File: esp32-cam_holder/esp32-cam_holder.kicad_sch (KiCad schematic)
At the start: 5 parts, among them J1 RJ45_Shielded, J2 Conn_01x03_Pin, U1 ESP32-CAM

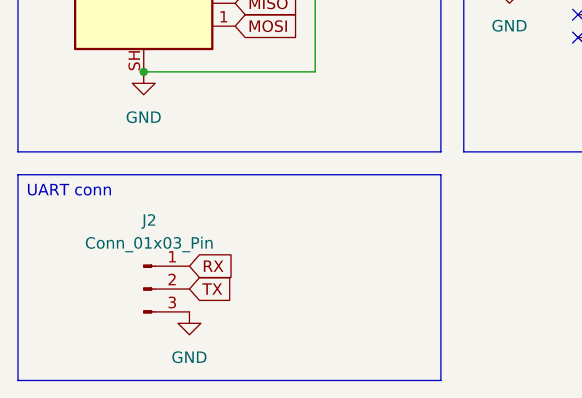
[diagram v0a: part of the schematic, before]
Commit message: update
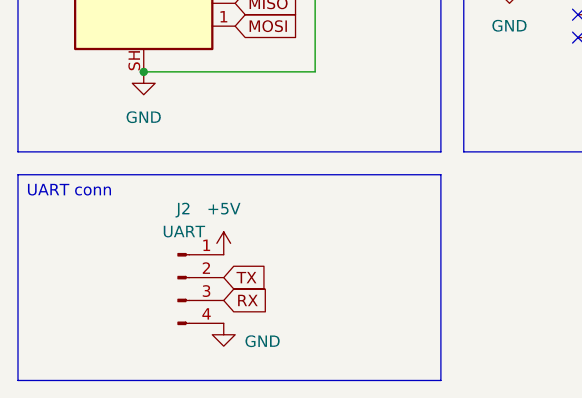
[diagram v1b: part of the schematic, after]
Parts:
- removed J2: Conn_01x03_Pin, Connector_PinHeader_2.54mm:PinHeader_1x03_P2.54mm_Horizontal, symbol Connector:Conn_01x03_Pin
- added J2: UART, Connector_PinHeader_2.54mm:PinHeader_1x04_P2.54mm_Horizontal, symbol Connector:Conn_01x04_Pin
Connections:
- net +5V: now also J2.1 (Pin_1)
- net GND: now also J2.4 (Pin_4)
- net RX: now also J2.3 (Pin_3)
- net TX: now also J2.2 (Pin_2)
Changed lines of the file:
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@@
+		)
+	)
+	(global_label "TX"
+		(shape input)
+		(at 36.83 71.12 0)
+		(fields_autoplaced yes)
+		(effects
+			(font
+				(size 1.27 1.27)
+			)
+			(justify left)
+		)
+		(property "Intersheetrefs" "${INTERSHEET_REFS}"
+			(at 41.9923 71.12 0)
+			(hide yes)
+			(show_name no)
+			(do_not_autoplace no)
+			(effects
+				(font
+					(size 1.27 1.27)
+				)
+				(justify left)
+			)
 		)
 	)
@@
 		)
 	)
-	(global_label "RX"
+	(global_label "MISO"
 		(shape input)
-		(at 33.02 69.85 0)
+		(at 38.1 40.64 0)
 		(fields_autoplaced yes)
 		(effects
@@
 		)
 		(property "Intersheetrefs" "${INTERSHEET_REFS}"
-			(at 38.4847 69.85 0)
+			(at 45.6814 40.64 0)
 			(hide yes)
 			(show_name no)
@@
 	(global_label "MISO"
 		(shape input)
-		(at 38.1 40.64 0)
+		(at 111.76 39.37 0)
 		(fields_autoplaced yes)
 		(effects
@@
 		)
 		(property "Intersheetrefs" "${INTERSHEET_REFS}"
-			(at 45.6814 40.64 0)
+			(at 119.3414 39.37 0)
 			(hide yes)
 			(show_name no)
@@
 		)
 	)
-	(global_label "MISO"
+	(global_label "TX"
 		(shape input)
-		(at 111.76 39.37 0)
+		(at 76.2 29.21 180)
 		(fields_autoplaced yes)
 		(effects
@@
 				(size 1.27 1.27)
 			)
-			(justify left)
+			(justify right)
 		)
 		(property "Intersheetrefs" "${INTERSHEET_REFS}"
-			(at 119.3414 39.37 0)
-			(hide yes)
-			(show_name no)
-			(do_not_autoplace no)
-			(effects
-				(font
-					(size 1.27 1.27)
-				)
-				(justify left)
-			)
-		)
-	)
-	(global_label "TX"
+			(at 71.0377 29.21 0)
+			(hide yes)
+			(show_name no)
+			(do_not_autoplace no)
+			(effects
+				(font
+					(size 1.27 1.27)
+				)
+				(justify right)
+			)
+		)
+	)
+	(global_label "RX"
 		(shape input)
-		(at 76.2 29.21 180)
+		(at 36.83 73.66 0)
 		(fields_autoplaced yes)
 		(effects
@@
 				(size 1.27 1.27)
 			)
-			(justify right)
+			(justify left)
 		)
 		(property "Intersheetrefs" "${INTERSHEET_REFS}"
-			(at 71.0377 29.21 0)
-			(hide yes)
-			(show_name no)
-			(do_not_autoplace no)
-			(effects
-				(font
-					(size 1.27 1.27)
-				)
-				(justify right)
+			(at 42.2947 73.66 0)
+			(hide yes)
+			(show_name no)
+			(do_not_autoplace no)
+			(effects
+				(font
+					(size 1.27 1.27)
+				)
+				(justify left)
 			)
 		)
@@
 		(property "Intersheetrefs" "${INTERSHEET_REFS}"
 			(at 126.0542 34.29 0)
-			(hide yes)
-			(show_name no)
-			(do_not_autoplace no)
-			(effects
-				(font
-					(size 1.27 1.27)
-				)
-				(justify left)
-			)
-		)
-	)
-	(global_label "TX"
-		(shape input)
-		(at 33.02 72.39 0)
-		(fields_autoplaced yes)
-		(effects
-			(font
-				(size 1.27 1.27)
-			)
-			(justify left)
-		)
-		(property "Intersheetrefs" "${INTERSHEET_REFS}"
-			(at 38.1823 72.39 0)
 			(hide yes)
 			(show_name no)
@@
 	)
 	(symbol
-		(lib_id "Connector:Conn_01x03_Pin")
-		(at 27.94 72.39 0)
+		(lib_id "Connector:Conn_01x04_Pin")
+		(at 31.75 71.12 0)
 		(unit 1)
 		(body_style 1)
@@
 		(fields_autoplaced yes)
 		(property "Reference" "J2"
-			(at 28.575 64.77 0)
-			(show_name no)
-			(do_not_autoplace no)
-			(effects
-				(font
-					(size 1.27 1.27)
-				)
-			)
-		)
-		(property "Value" "Conn_01x03_Pin"
-			(at 28.575 67.31 0)
-			(show_name no)
-			(do_not_autoplace no)
-			(effects
-				(font
-					(size 1.27 1.27)
-				)
-			)
-		)
-		(property "Footprint" "Connector_PinHeader_2.54mm:PinHeader_1x03_P2.54mm_Horizontal"
-			(at 27.94 72.39 0)
+			(at 32.385 63.5 0)
+			(show_name no)
+			(do_not_autoplace no)
+			(effects
+				(font
+					(size 1.27 1.27)
+				)
+			)
+		)
+		(property "Value" "UART"
+			(at 32.385 66.04 0)
+			(show_name no)
+			(do_not_autoplace no)
+			(effects
+				(font
+					(size 1.27 1.27)
+				)
+			)
+		)
+		(property "Footprint" "Connector_PinHeader_2.54mm:PinHeader_1x04_P2.54mm_Horizontal"
+			(at 31.75 71.12 0)
 			(hide yes)
 			(show_name no)
@@
 		)
 		(property "Datasheet" ""
-			(at 27.94 72.39 0)
-			(hide yes)
-			(show_name no)
-			(do_not_autoplace no)
-			(effects
-				(font
-					(size 1.27 1.27)
-				)
-			)
-		)
-		(property "Description" "Generic connector, single row, 01x03, script generated"
-			(at 27.94 72.39 0)
-			(hide yes)
-			(show_name no)
-			(do_not_autoplace no)
-			(effects
-				(font
-					(size 1.27 1.27)
-				)
-			)
+			(at 31.75 71.12 0)
+			(hide yes)
+			(show_name no)
+			(do_not_autoplace no)
+			(effects
+				(font
+					(size 1.27 1.27)
+				)
+			)
+		)
+		(property "Description" "Generic connector, single row, 01x04, script generated"
+			(at 31.75 71.12 0)
+			(hide yes)
+			(show_name no)
+			(do_not_autoplace no)
+			(effects
+				(font
+					(size 1.27 1.27)
+				)
+			)
+		)
+		(pin "4"
+		)
+		(pin "1"
 		)
 		(pin "2"
-		)
-		(pin "1"
 		)
 		(pin "3"
@@
 	)
 	(symbol
+		(lib_id "power:+5V")
+		(at 36.83 68.58 0)
+		(unit 1)
+		(body_style 1)
+		(exclude_from_sim no)
+		(in_bom yes)
+		(on_board yes)
+		(in_pos_files yes)
+		(dnp no)
+		(fields_autoplaced yes)
+		(property "Reference" "#PWR06"
+			(at 36.83 72.39 0)
+			(hide yes)
+			(show_name no)
+			(do_not_autoplace no)
+			(effects
+				(font
+					(size 1.27 1.27)
+				)
+			)
+		)
+		(property "Value" "+5V"
+			(at 36.83 63.5 0)
+			(show_name no)
+			(do_not_autoplace no)
+			(effects
+				(font
+					(size 1.27 1.27)
+				)
+			)
+		)
+		(property "Footprint" ""
+			(at 36.83 68.58 0)
+			(hide yes)
+			(show_name no)
+			(do_not_autoplace no)
+			(effects
+				(font
+					(size 1.27 1.27)
+				)
+			)
+		)
+		(property "Datasheet" ""
+			(at 36.83 68.58 0)
+			(hide yes)
+			(show_name no)
+			(do_not_autoplace no)
+			(effects
+				(font
+					(size 1.27 1.27)
+				)
+			)
+		)
+		(property "Description" "Power symbol creates a global label with name \"+5V\""
+			(at 36.83 68.58 0)
+			(hide yes)
+			(show_name no)
+			(do_not_autoplace no)
+			(effects
+				(font
+					(size 1.27 1.27)
+				)
+			)
+		)
+		(pin "1"
+		)
+		(instances
+			(project "esp32-cam_holder"
+				(path "/a446d434-d129-49bb-b3ed-ecea04be15d0"
+					(reference "#PWR06")
+					(unit 1)
+				)
+			)
+		)
+	)
+	(symbol
 		(lib_id "Connector:RJ45_Shielded")
 		(at 27.94 35.56 0)
@@
 	(symbol
 		(lib_id "power:GND")
-		(at 33.02 74.93 0)
+		(at 36.83 76.2 0)
 		(unit 1)
 		(body_style 1)
@@
 		(in_pos_files yes)
 		(dnp no)
-		(fields_autoplaced yes)
 		(property "Reference" "#PWR05"
-			(at 33.02 81.28 0)
+			(at 36.83 82.55 0)
 			(hide yes)
 			(show_name no)
@@
 		)
 		(property "Value" "GND"
-			(at 33.02 80.01 0)
+			(at 41.148 78.232 0)
 			(show_name no)
 			(do_not_autoplace no)
@@
 		)
 		(property "Footprint" ""
-			(at 33.02 74.93 0)
+			(at 36.83 76.2 0)
 			(hide yes)
 			(show_name no)
@@
 		)
 		(property "Datasheet" ""
-			(at 33.02 74.93 0)
+			(at 36.83 76.2 0)
 			(hide yes)
 			(show_name no)
@@
 		)
 		(property "Description" "Power symbol creates a global label with name \"GND\" , ground"
-			(at 33.02 74.93 0)
-			(hide yes)
-			(show_name no)
+			(at 36.83 76.2 0)
+			(hide yes)
+			(show_name no)
